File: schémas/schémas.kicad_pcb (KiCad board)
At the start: 2 copper layers, 46 x 40.5 mm, 7 parts, among them J2 Conn_01x04, J3 Conn_01x08, J4 Conn_01x08, J5 Conn_01x03, SW3 SW_Push

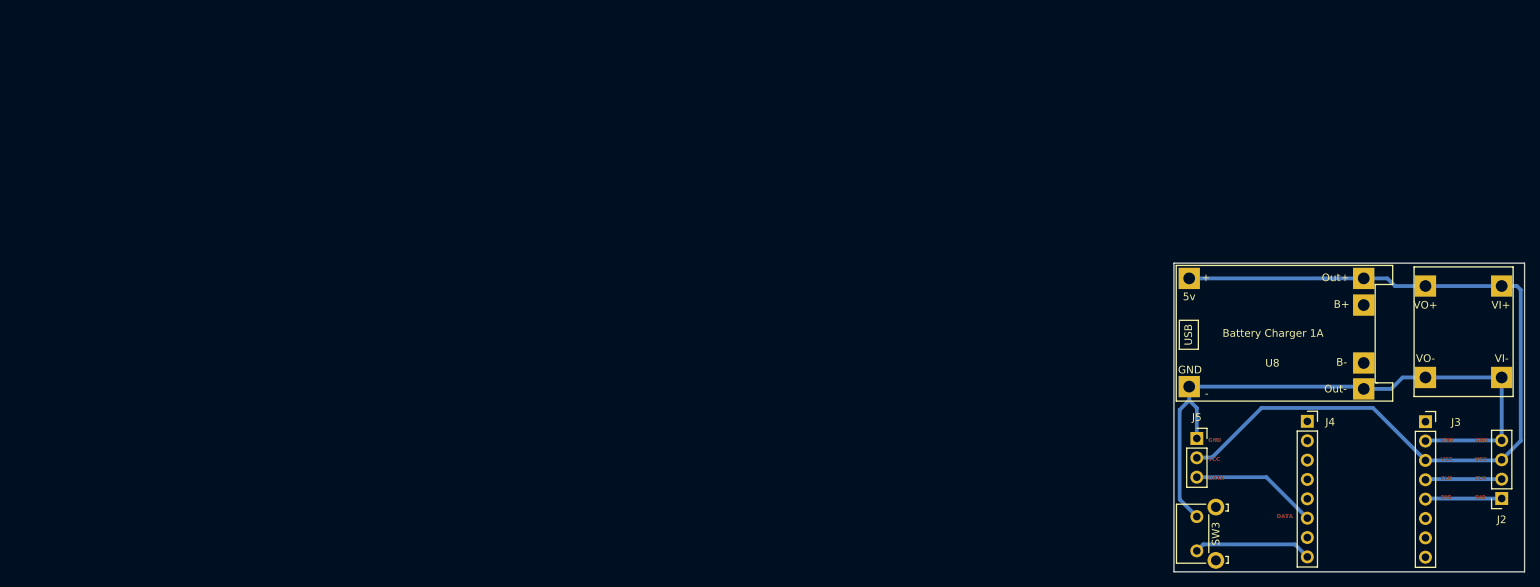
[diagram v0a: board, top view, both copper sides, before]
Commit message: feat: changed schemas
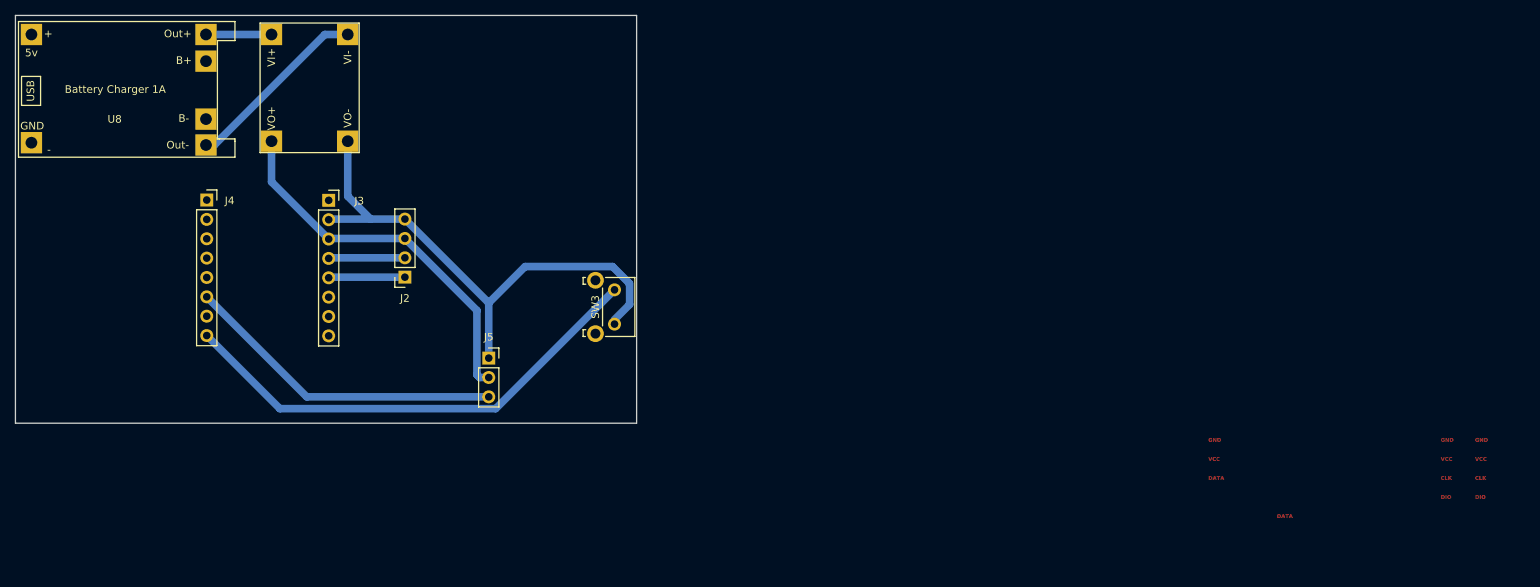
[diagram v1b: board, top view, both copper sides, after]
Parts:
- moved U9 159.1 mm to (57.6, 13.5), turned to -90 degrees
- moved U8 155.2 mm to (12.9, 13.3)
- moved J4 147.3 mm to (37.6, 36.7)
- moved J2 146.8 mm to (63.6, 46.8)
- moved J3 146.8 mm to (53.6, 36.8)
- moved J5 93.5 mm to (74.6, 57.5)
- moved SW3 83.7 mm to (91.1, 48.5), turned to -90 degrees
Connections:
- U8 pad 1: +3.3V -> unconnected-(U8-IN+-Pad1)
- U8 pad 2: GND -> unconnected-(U8-IN--Pad2)
- U8 pad 3: +3.3V -> Net-(U8-OUT+)
- U8 pad 4: GND -> Net-(U8-OUT-)
- U9 pad 1: GND -> Net-(U8-OUT-)
- U9 pad 2: +3.3V -> Net-(U8-OUT+)
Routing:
- net +3.3V: track 113.0 -> 49.5 mm
- net Net-(J4-Pin_8): track 15.5 -> 63.9 mm
- net Net-(U8-OUT-): track 0.00 -> 26.3 mm
- net Net-(J4-Pin_6): track 16.7 -> 42.4 mm
- net GND: track 84.5 -> 71.2 mm
- net Net-(U8-OUT+): track 0.00 -> 8.60 mm
- net unconnected-(U8-IN--Pad2): track 0.00 -> 1.13 mm
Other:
- board size 46 x 40.5 mm -> 81.5 x 53.5 mm
